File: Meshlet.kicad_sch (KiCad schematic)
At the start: 102 parts, among them J11 GPIO Exp., J12 GPS Header, J13 Thermistor Pins, J14 Ext. Notif. Header, J2 User Btn Header, J3 Batt. Header (Picoblade 1.25), J4 Batt. Header (JST-PH 2.0), J5 USB_C_Receptacle_USB2.0_16P, J6 I2C Header, J7 Ext. Power Header, J9 Ext. Power Header, Q1 AO3400A, SW2 BOOTSEL, U1 XC6206PxxxMR, U11 INA3221, U2 USBLC6-2SC6, U3 XC6206PxxxMR, U4 RP2350_60QFN, U5 Wio-SX1262, U6 BQ25185, U7 BME280, U8 W25Q32JVZP, U9 XC6206PxxxMR, Y1 12.000MHz

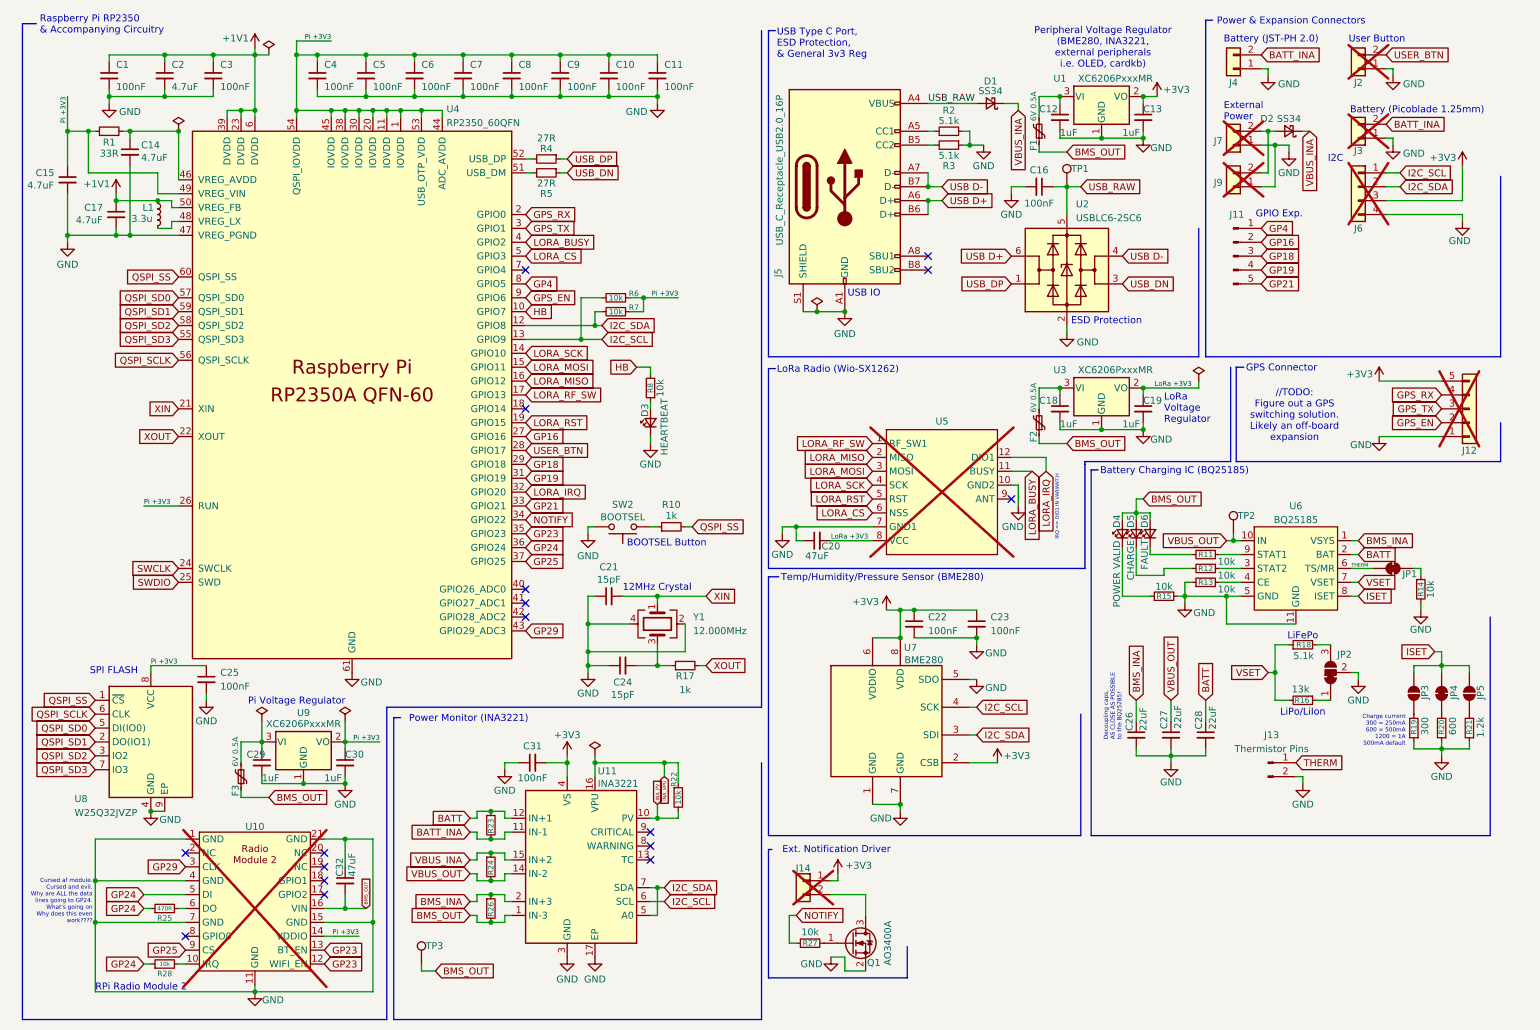
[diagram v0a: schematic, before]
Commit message: ibom updates
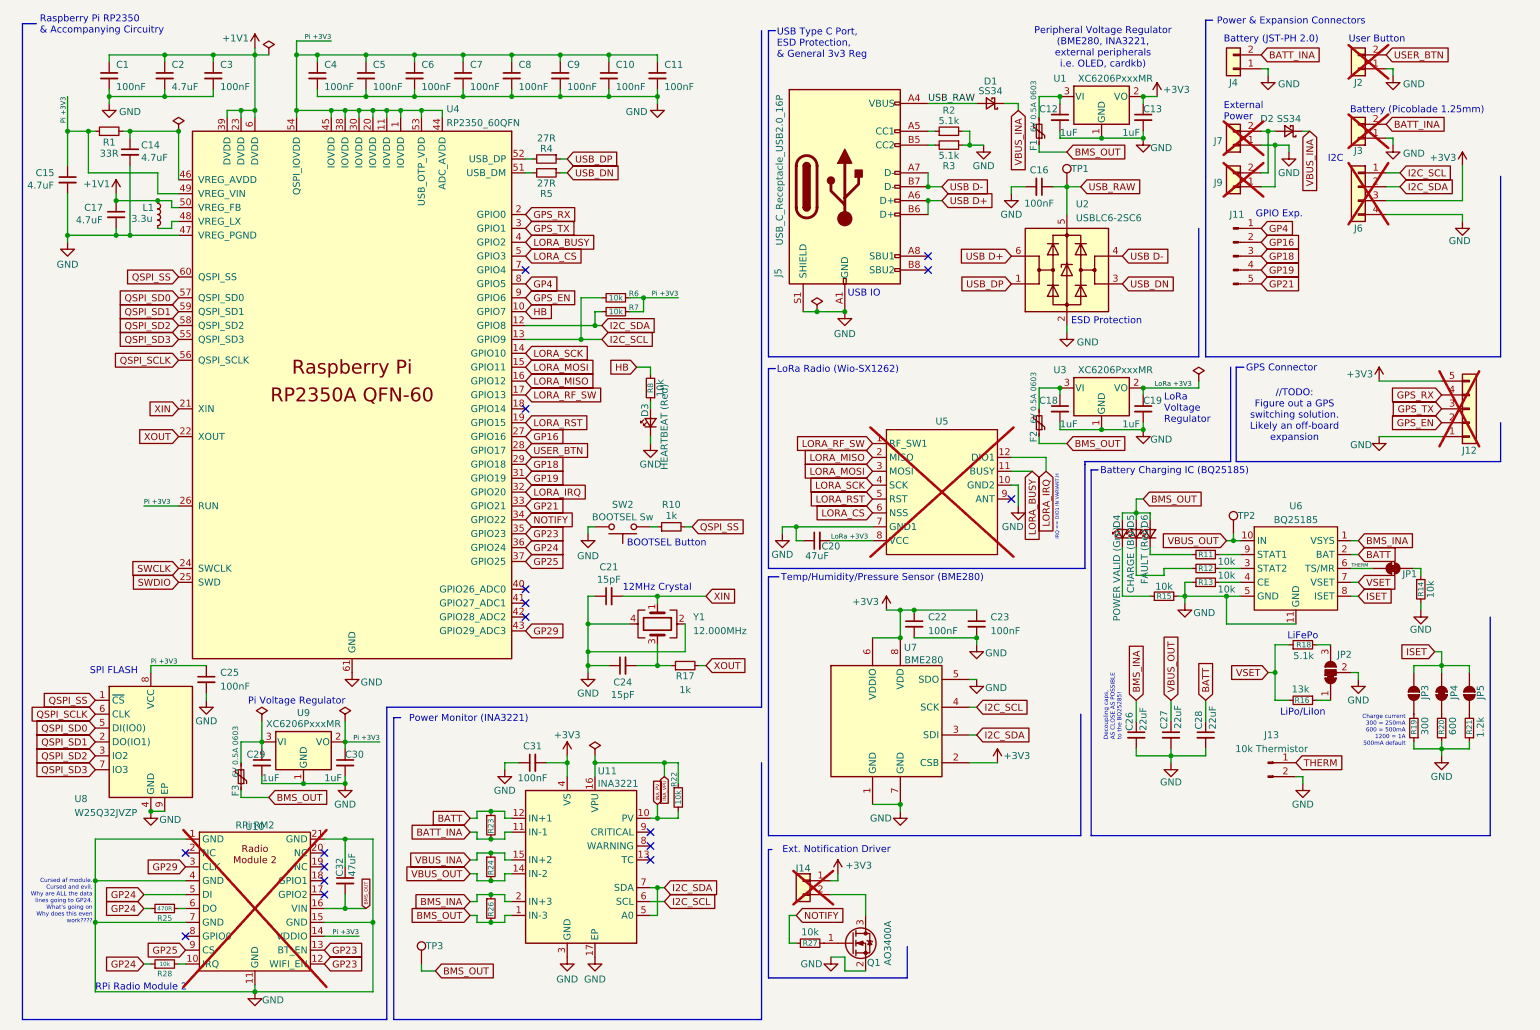
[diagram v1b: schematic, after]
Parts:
- D3: value HEARTBEAT -> HEARTBEAT (Red)
- D4: value POWER VALID -> POWER VALID (Grn)
- D5: value CHARGE -> CHARGE (Blu)
- D6: value FAULT -> FAULT (Red)
- F1, F2, F3: value 6V 0.5A -> 6V 0.5A 0603
- J13: value Thermistor Pins -> 10k Thermistor
- JP3: value SolderJumper_2_Open -> 250mA Charge
- JP4: value SolderJumper_2_Bridged -> 500mA Charge
- JP5: value SolderJumper_2_Open -> 1A Charge
- SW2: value BOOTSEL -> BOOTSEL Sw
- U10: value ~ -> RPi RM2
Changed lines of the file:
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@@
 			)
 		)
-		(property "Value" "Thermistor Pins"
+		(property "Value" "10k Thermistor"
 			(at 241.935 147.32 0)
 			(effects
@@
 			)
 		)
-		(property "Value" "POWER VALID"
+		(property "Value" "POWER VALID (Grn)"
 			(at 213.614 115.316 0)
 			(effects
@@
 			)
 		)
-		(property "Value" "CHARGE"
+		(property "Value" "CHARGE (Blu)"
 			(at 216.154 112.776 0)
 			(effects
@@
 			)
 		)
-		(property "Value" "SolderJumper_2_Bridged"
+		(property "Value" "500mA Charge"
 			(at 275.59 138.4299 90)
 			(effects
@@
 			)
 		)
-		(property "Value" "6V 0.5A"
+		(property "Value" "6V 0.5A 0603"
 			(at 198.374 29.718 90)
 			(effects
@@
 			)
 		)
-		(property "Value" "HEARTBEAT"
+		(property "Value" "HEARTBEAT (Red)"
 			(at 130.81 88.392 0)
 			(effects
@@
 			)
 		)
-		(property "Value" "6V 0.5A"
+		(property "Value" "6V 0.5A 0603"
 			(at 52.324 147.828 90)
 			(effects
@@
 			)
 		)
-		(property "Value" "6V 0.5A"
+		(property "Value" "6V 0.5A 0603"
 			(at 198.374 83.058 90)
 			(effects
@@
 			)
 		)
-		(property "Value" "BOOTSEL"
+		(property "Value" "BOOTSEL Sw"
 			(at 123.19 104.902 0)
 			(effects
@@
 			)
 		)
-		(property "Value" "FAULT"
+		(property "Value" "FAULT (Red)"
 			(at 218.694 111.76 0)
 			(effects
@@
 			)
 		)
-		(property "Value" "SolderJumper_2_Open"
+		(property "Value" "250mA Charge"
 			(at 270.51 138.4299 90)
 			(effects
@@
 			)
 		)
-		(property "Value" "~"
+		(property "Value" "RPi RM2"
 			(at 55.88 161.29 0)
 			(effects
@@
 			)
 		)
-		(property "Value" "SolderJumper_2_Open"
+		(property "Value" "1A Charge"
 			(at 280.67 138.4299 90)
 			(effects
